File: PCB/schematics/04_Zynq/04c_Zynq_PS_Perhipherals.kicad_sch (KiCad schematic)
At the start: 151 parts, among them J1 HR911105A_C12074, J10 Conn_02x07_Odd_Even, J11 Conn_01x04_Pin, J3 USB3_B, J6 3.3V_I2C, U28 TXS02612RTWR, U29 MT25QU256ABA8ESF-0SIT TR, U30 FEMDNN032G-A3A55, U31 DP83867IRRGZR, U32 CP2102N-A02-GQFN24, U33 USB3320C-EZK-TR, U34 TPD4E05U06DQA, U35 TCA9548APWR, U36 TXB0108PW, U37 PCA9306, U38 USB2514B_Bi, U53 TCA9548APWR, Y1 25 MHz, Y2 25 MHz, Y3 26 MHz

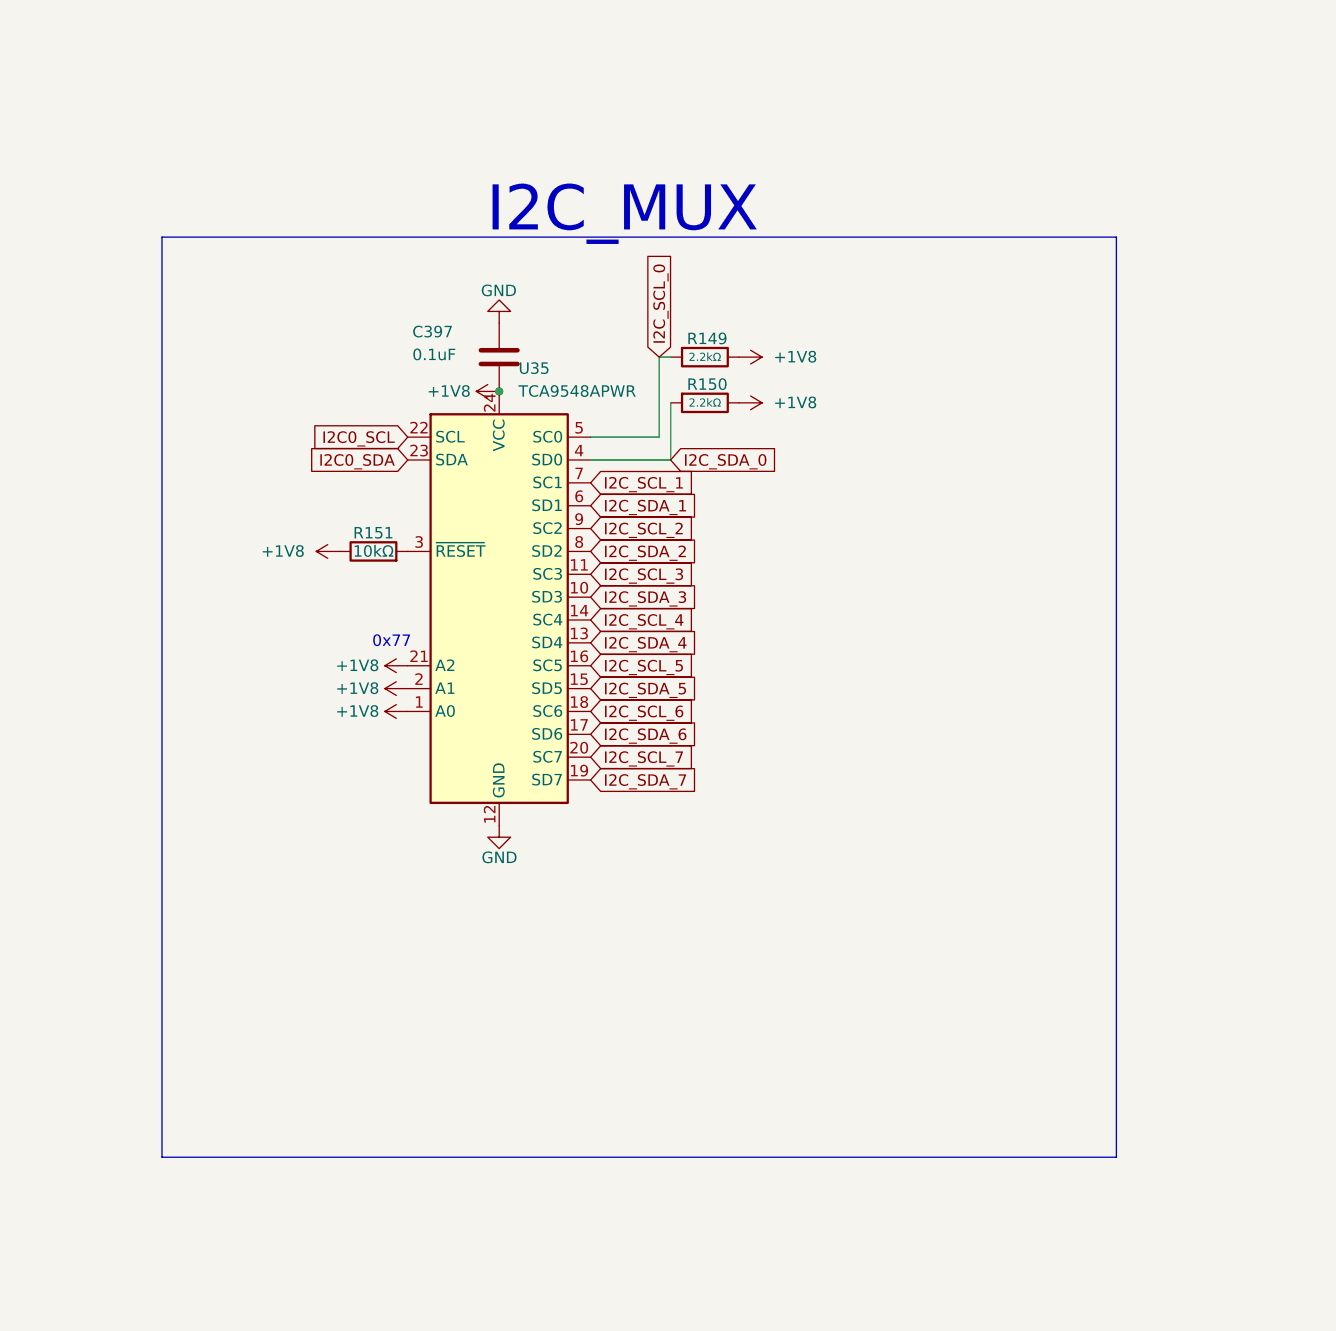
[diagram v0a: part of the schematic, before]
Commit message: Feat : Finished four sections of Placement
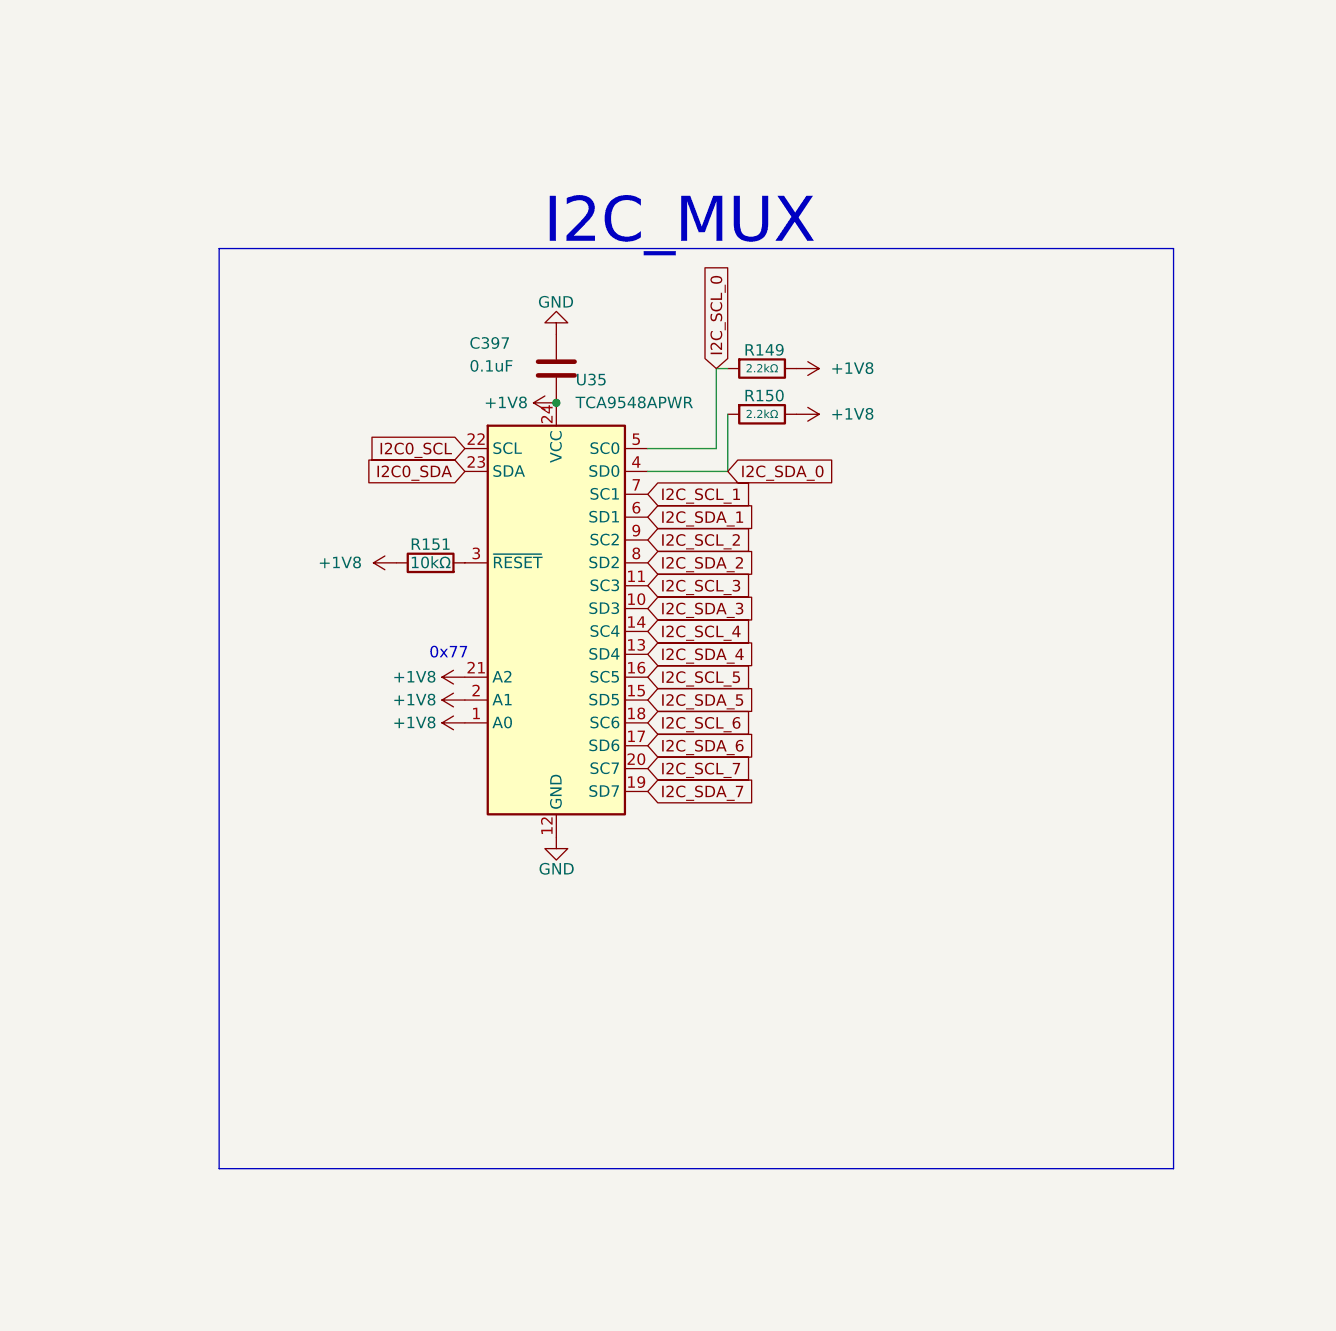
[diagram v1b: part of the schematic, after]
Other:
- moved on the sheet: C397, R149, R150, R151, U35
